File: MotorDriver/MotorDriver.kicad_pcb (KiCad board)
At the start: 2 copper layers, 78 x 48.6 mm, 47 parts, among them J1 VIN, J2 INPUT, M1 Motor_DC, Q1 Q_NMOS_GDS, Q2 Q_NMOS_GDS, Q3 Q_NMOS_GDS, Q4 Q_NMOS_GDS, U1 IR2302, U2 IR2302, U3 74HC00, U4 TLP2348, U5 TLP2348, U6 NJM7812SDL1

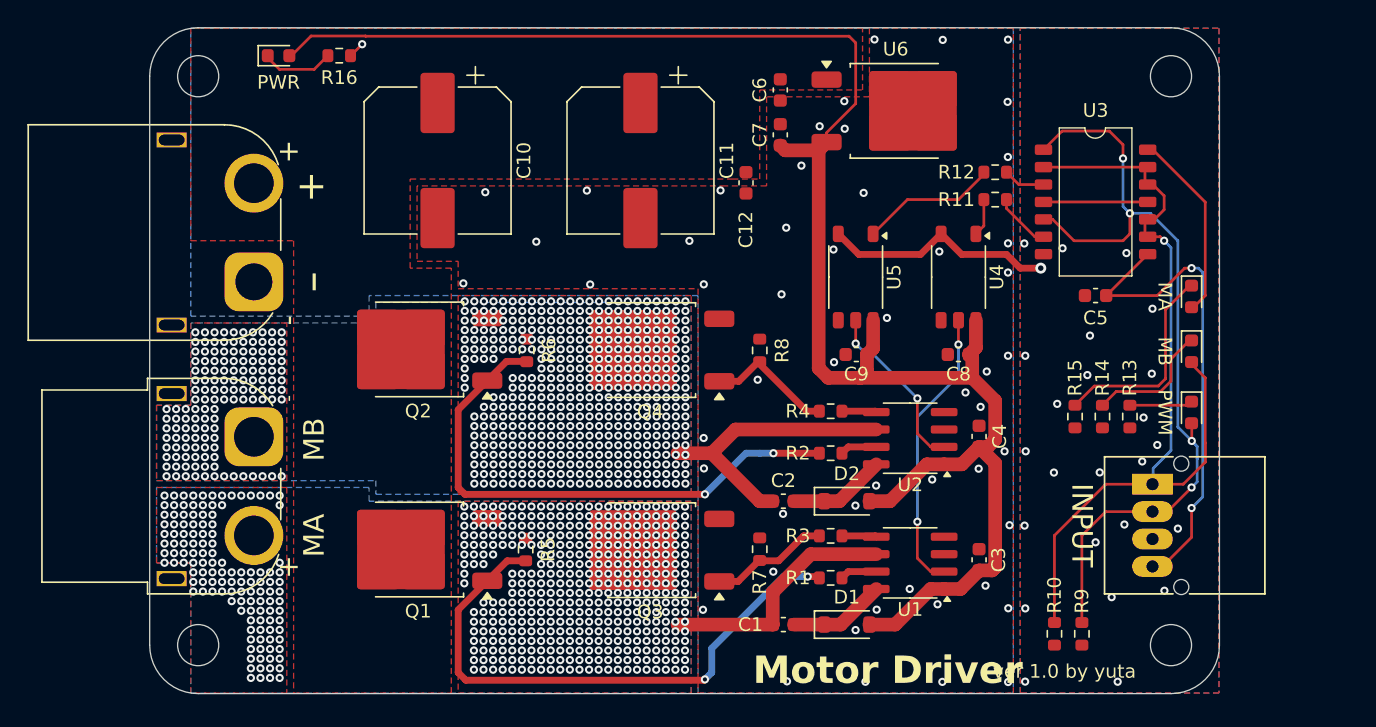
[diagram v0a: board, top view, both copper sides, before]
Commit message: Motor Driver ver2.0
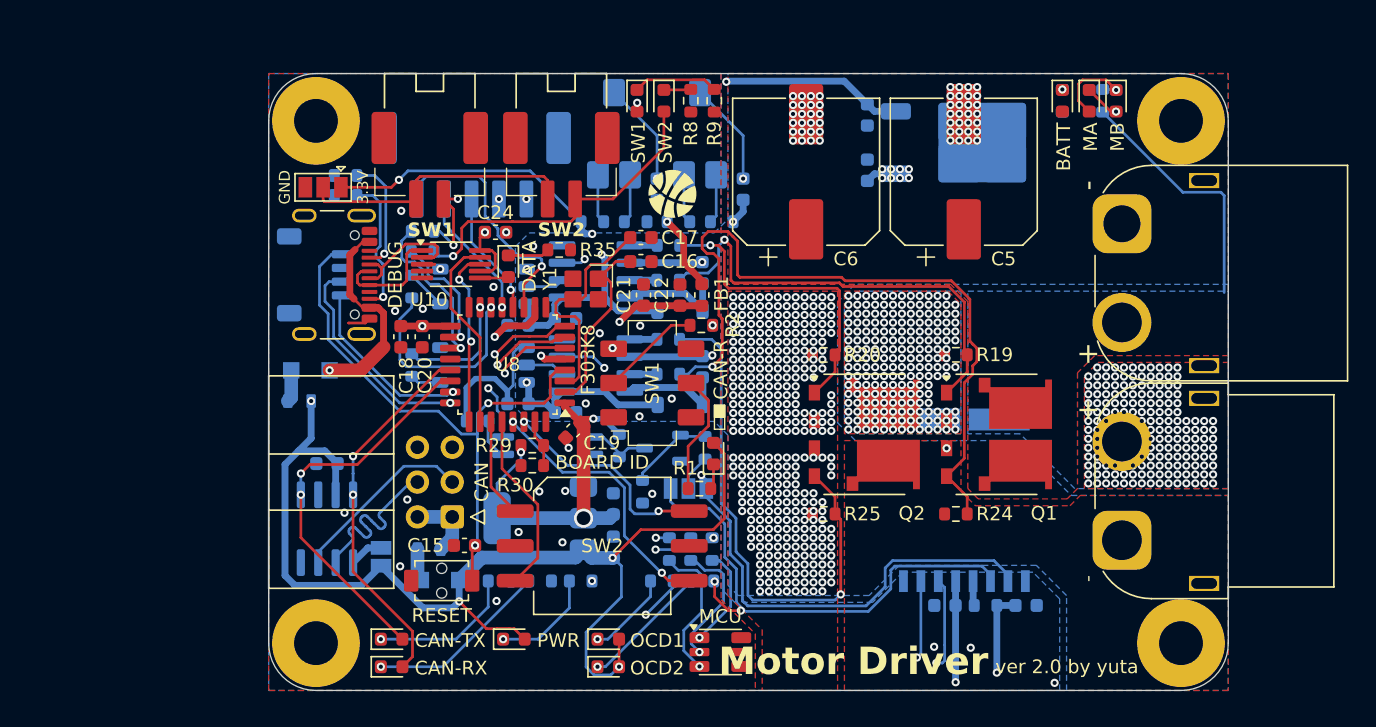
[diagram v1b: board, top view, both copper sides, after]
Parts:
- removed M1: Motor_DC, Anan-Robo_Footprint_Library:XT60PW-F_Horizontal
- removed Q4: Q_NMOS_GDS, Package_TO_SOT_SMD:TO-252-2
- added C13: 2.5u, Capacitor_SMD:C_0603_1608Metric, B.Cu at (150.1, 100.5)
- added C14: 0.1u, Capacitor_SMD:C_0603_1608Metric, B.Cu at (140.2, 103.8)
- added C15: 0.1u, Capacitor_SMD:C_0603_1608Metric, F.Cu at (132.8, 113.5)
- added C16: 15p, Capacitor_SMD:C_0603_1608Metric, F.Cu at (145.7, 92.8)
- added C17: 15p, Capacitor_SMD:C_0603_1608Metric, F.Cu at (145.7, 91.1)
- added C18: 4.7u, Capacitor_SMD:C_0603_1608Metric, F.Cu at (128.1, 98.3)
- added C19: 0.1u, Capacitor_SMD:C_0603_1608Metric, F.Cu at (140.7, 105.2)
- added C20: 0.1u, Capacitor_SMD:C_0603_1608Metric, F.Cu at (129.7, 98.3)
- added C21: 0.1u, Capacitor_SMD:C_0603_1608Metric, F.Cu at (145.8, 95.3)
- added C22: 1u, Capacitor_SMD:C_0603_1608Metric, F.Cu at (148.5, 95.3)
- added C23: 0.1u, Capacitor_SMD:C_0603_1608Metric, B.Cu at (122.8, 107.6)
- added C24: 0.1u, Capacitor_SMD:C_0603_1608Metric, F.Cu at (135.1, 90.7)
- added C25: 0.1u, Capacitor_SMD:C_0603_1608Metric, B.Cu at (136.7, 97.5)
- added C26: 0.1u, Capacitor_SMD:C_0603_1608Metric, B.Cu at (136.7, 103.2)
- added D10: OCD1, LED_SMD:LED_0603_1608Metric, F.Cu at (143.3, 120.4)
- added D11: OCD2, LED_SMD:LED_0603_1608Metric, F.Cu at (143.3, 122.4)
- added D12: D_Schottky, Diode_SMD:D_SOD-123, B.Cu at (148.5, 103.3)
- added D13: CAN_TX, LED_SMD:LED_0603_1608Metric, F.Cu at (127.5, 120.4)
- added D14: CAN_RX, LED_SMD:LED_0603_1608Metric, F.Cu at (127.5, 122.4)
- added D15: D, Diode_SMD:Nexperia_CFP3_SOD-123W, B.Cu at (121.5, 100.8)
- added D16: DATA, LED_SMD:LED_0603_1608Metric, F.Cu at (136.0, 93.2)
- added D7: D_Schottky, Diode_SMD:D_SOD-123, B.Cu at (148.5, 96.4)
- added D8: MA, LED_SMD:LED_0603_1608Metric, F.Cu at (178.4, 81.1)
- added D9: MB, LED_SMD:LED_0603_1608Metric, F.Cu at (180.3, 81.1)
- added F1: Polyfuse, Anan-Robo_Footprint_Library:MF-FSMF, B.Cu at (130.2, 113.8)
- added F2: Polyfuse, Anan-Robo_Footprint_Library:MF-FSMF, B.Cu at (120.7, 103.0)
- added FB1: FerriteBead, Inductor_SMD:L_0603_1608Metric, F.Cu at (150.1, 95.3)
- added G***: LOGO, LOGO, F.Cu at (147.9, 87.9)
- added H1: MountingHole_Pad, MountingHole:MountingHole_3.2mm_M3_Pad, F.Cu at (122.0, 82.6)
- added H2: MountingHole_Pad, MountingHole:MountingHole_3.2mm_M3_Pad, F.Cu at (122.0, 120.7)
- added H3: MountingHole_Pad, MountingHole:MountingHole_3.2mm_M3_Pad, F.Cu at (185.1, 82.6)
- added H4: MountingHole_Pad, MountingHole:MountingHole_3.2mm_M3_Pad, F.Cu at (185.1, 120.7)
- added H5: MountingHole, Anan-Robo_Footprint_Library:Title, F.Cu at (77.9, 108.2)
- added H6: MountingHole, Anan-Robo_Footprint_Library:Aho_old_S, B.Cu at (169.9, 94.6)
- added H7: MountingHole, Anan-Robo_Footprint_Library:Aho_new_S, B.Cu at (158.4, 94.6)
- added H8: MountingHole, Anan-Robo_Footprint_Library:Info_M_3, B.Cu at (158.4, 107.3)
- added J3: SW1, Anan-Robo_Footprint_Library:SM02B-PASS-TBx, F.Cu at (130.2, 84.4)
- added J4: SW2, Anan-Robo_Footprint_Library:SM02B-PASS-TBx, F.Cu at (139.8, 84.4)
- added J5: VIN, Anan-Robo_Footprint_Library:XT60PW-M_Horizontal, F.Cu at (189.5, 93.8)
- added J6: Motor, Anan-Robo_Footprint_Library:XT60PW-F_Horizontal, F.Cu at (186.7, 109.8)
- added J7: SWD, Connector_JST:JST_SH_SM04B-SRSS-TB_1x04-1MP_P1.00mm_Horizontal, B.Cu at (121.9, 93.8)
- added J8: Debug, Connector_USB:USB_C_Receptacle_GCT_USB4105-xx-A_16P_TopMnt_Horizontal, F.Cu at (122.2, 93.8)
- added JP1: Up/Down, Jumper:SolderJumper-3_P1.3mm_Open_Pad1.0x1.5mm, F.Cu at (122.5, 87.4)
- added JP2: OCD, Jumper:SolderJumper-3_P1.3mm_Open_Pad1.0x1.5mm, B.Cu at (149.1, 109.4)
- added JP4: MCP2561/2FD selector, Jumper:SolderJumper-2_P1.3mm_Open_Pad1.0x1.5mm, B.Cu at (126.7, 114.4)
- added R17: 80, Resistor_SMD:R_0603_1608Metric, B.Cu at (147.7, 91.7)
- added R18: 1.5k, Resistor_SMD:R_0603_1608Metric, B.Cu at (170.8, 117.9)
- added R19: 10k, Resistor_SMD:R_0603_1608Metric, F.Cu at (168.6, 99.6)
- added R20: 10k, Resistor_SMD:R_0603_1608Metric, F.Cu at (159.0, 99.7)
- added R21: 3.7k, Resistor_SMD:R_0603_1608Metric, B.Cu at (179.3, 81.1)
- added R22: 420, Resistor_SMD:R_0603_1608Metric, B.Cu at (147.2, 116.1)
- added R23: 420, Resistor_SMD:R_0603_1608Metric, B.Cu at (150.1, 116.1)
- added R24: 10k, Resistor_SMD:R_0603_1608Metric, F.Cu at (168.6, 111.2)
- added R25: 10k, Resistor_SMD:R_0603_1608Metric, F.Cu at (159.0, 111.2)
- added R26: 80, Resistor_SMD:R_0603_1608Metric, B.Cu at (147.7, 101.1)
- added R27: 80, Resistor_SMD:R_0603_1608Metric, B.Cu at (147.6, 98.5)
- added R28: 1k, Resistor_SMD:R_0603_1608Metric, B.Cu at (144.1, 106.3)
- added R29: 10k, Resistor_SMD:R_0603_1608Metric, F.Cu at (137.7, 106.3)
- added R30: 10k, Resistor_SMD:R_0603_1608Metric, F.Cu at (137.7, 107.7)
- added R31: 100, Resistor_SMD:R_0603_1608Metric, B.Cu at (135.3, 116.1)
- added R32: 100, Resistor_SMD:R_0603_1608Metric, B.Cu at (138.3, 116.1)
- added R33: 5.1k, Resistor_SMD:R_0603_1608Metric, B.Cu at (124.1, 88.0)
- added R34: 5.1k, Resistor_SMD:R_0603_1608Metric, B.Cu at (124.1, 86.6)
- added R35: 100, Resistor_SMD:R_0603_1608Metric, F.Cu at (139.7, 92.0)
- added R36: 350, Resistor_SMD:R_0603_1608Metric, B.Cu at (128.9, 94.7)
- added R37: 350, Resistor_SMD:R_0603_1608Metric, B.Cu at (128.9, 100.4)
- added R38: 660, Resistor_SMD:R_0603_1608Metric, B.Cu at (150.3, 106.4)
- added R39: 10k, Resistor_SMD:R_0603_1608Metric, B.Cu at (145.8, 109.6)
- added R40: 10k, Resistor_SMD:R_0603_1608Metric, B.Cu at (133.7, 104.5)
- added RV1: 10k, Anan-Robo_Footprint_Library:ST-4ETB103, B.Cu at (150.0, 83.5)
- added RV2: 10k, Anan-Robo_Footprint_Library:ST-4ETB103, B.Cu at (143.7, 83.5)
- added SW1: CAN_R, Anan-Robo_Footprint_Library:SLW, F.Cu at (146.5, 101.7)
- added SW2: SW_Coded, Anan-Robo_Footprint_Library:RDS-1055-SMT, F.Cu at (142.8, 113.6)
- added SW3: RESET, Anan-Robo_Footprint_Library:TVAF06-A020B-R, F.Cu at (131.1, 116.1)
- added U10: CH340E, Package_SO:MSOP-10_3x3mm_P0.5mm, F.Cu at (131.8, 93.0)
- added U11: TLP2348, Package_SO:SO-5-6_4.55x3.7mm_P1.27mm, B.Cu at (134.2, 94.7)
- added U12: TLP2348, Package_SO:SO-5-6_4.55x3.7mm_P1.27mm, B.Cu at (134.2, 100.4)
- added U7: TLP293, Package_SO:SOIC-4_4.55x2.6mm_P1.27mm, B.Cu at (138.8, 106.3)
- added U8: STM32F303K8Tx, Package_QFP:LQFP-32_7x7mm_P0.8mm, F.Cu at (135.9, 100.3)
- added U9: MCP2561/2FD, Package_SO:SOIC-8_3.9x4.9mm_P1.27mm, B.Cu at (122.8, 112.3)
- added Y1: Crystal_GND2, Anan-Robo_Footprint_Library:XRCGB, F.Cu at (141.6, 94.8)
- C1: value 10u -> 0.33u; moved to B.Cu
- C10: value 330u -> 2.5u; footprint Capacitor_SMD:CP_Elec_10x10.5 -> Capacitor_SMD:C_0603_1608Metric; moved to B.Cu
- C11: value 330u -> 1000p; footprint Capacitor_SMD:CP_Elec_10x10.5 -> Capacitor_SMD:C_0603_1608Metric; moved to B.Cu
- C12: value 1u -> 1000p; moved to B.Cu
- C2: value 10u -> 4.7u; moved to B.Cu
- C3, C7, C9: moved to B.Cu
- C4: value 0.1u -> 4.7u; moved to B.Cu
- C5: value 0.1u -> 330u; footprint Capacitor_SMD:C_0603_1608Metric -> Capacitor_SMD:CP_Elec_10x10.5
- C6: value 0.33u -> 330u; footprint Capacitor_SMD:C_0603_1608Metric -> Capacitor_SMD:CP_Elec_10x10.5
- C8: value 0.1u -> 1000p; moved to B.Cu
- D1: value D_Schottky -> D; footprint Diode_SMD:D_SOD-123 -> Diode_SMD:Nexperia_CFP3_SOD-123W; moved to B.Cu
- D2: value D_Schottky -> CAN_R; footprint Diode_SMD:D_SOD-123 -> LED_SMD:LED_0603_1608Metric
- D3: value PWM -> SW2
- D4: value MA -> SW1
- D5: value MB -> PWR
- D6: value PWR -> BATT
- J1: value VIN -> CAN; footprint Anan-Robo_Footprint_Library:XT60PW-M_Horizontal -> Connector_IDC:IDC-Header_2x03_P2.54mm_Horizontal
- J2: value INPUT -> ENC; footprint Anan-Robo_Footprint_Library:PAコネクタ(4ピンサイド型) -> Anan-Robo_Footprint_Library:SM05B-PASS-TBx; moved to B.Cu
- Q1, Q2: value Q_NMOS_GDS -> Q_NMOS; footprint Package_TO_SOT_SMD:TO-252-2 -> Anan-Robo_Footprint_Library:Vishay_PowerPAK_8x8L_Dual
- Q3: value Q_NMOS_GDS -> Q_NMOS_GSD; footprint Package_TO_SOT_SMD:TO-252-2 -> Package_TO_SOT_SMD:TSOT-23; moved to B.Cu
- R1: value 80 -> 420
- R10: value 20k -> 430; moved to B.Cu
- R11: value 175 -> 1.5k; moved to B.Cu
- R12: value 175 -> 13k; moved to B.Cu
- R13: value 80 -> 2.4k; moved to B.Cu
- R14: value 80 -> 18k; moved to B.Cu
- R15: value 80 -> 3k; moved to B.Cu
- R16: value 500 -> 80; moved to B.Cu
- R2: value 80 -> 120
- R3: value 80 -> 100; moved to B.Cu
- R4: value 80 -> 600; moved to B.Cu
- R5: value 20k -> 300; moved to B.Cu
- R6, R7: value 20k -> 330; moved to B.Cu
- R8, R9: value 20k -> 80
- U1: value IR2302 -> LED_GRB; footprint Package_SO:SOIC-8_3.9x4.9mm_P1.27mm -> LED_SMD:LED_ROHM_SMLVN6
- U2: value IR2302 -> NJM7812SDL1; footprint Package_SO:SOIC-8_3.9x4.9mm_P1.27mm -> Package_TO_SOT_SMD:TO-252-2; moved to B.Cu
- U3: value 74HC00 -> TLV1117-33; footprint Anan-Robo_Footprint_Library:SOP14 -> Package_TO_SOT_SMD:SOT-223-3_TabPin2; moved to B.Cu
- U4: value TLP2348 -> CZ-3A05; footprint Package_SO:SO-5-6_4.55x3.7mm_P1.27mm -> Anan-Robo_Footprint_Library:CZ3A; moved to B.Cu
- U5: value TLP2348 -> IR2302; footprint Package_SO:SO-5-6_4.55x3.7mm_P1.27mm -> Package_SO:SOIC-8_3.9x4.9mm_P1.27mm; moved to B.Cu
- U6: value NJM7812SDL1 -> IR2302; footprint Package_TO_SOT_SMD:TO-252-2 -> Package_SO:SOIC-8_3.9x4.9mm_P1.27mm; moved to B.Cu
- moved J2 57.3 mm to (133.3, 83.6), turned to 180 degrees
- moved D6 57.3 mm to (176.4, 81.1), turned to -90 degrees
- moved D5 53.7 mm to (136.4, 120.4), turned to 0 degrees
- moved U3 50.4 mm to (138.3, 111.6), turned to 180 degrees
- moved R9 47.2 mm to (151.0, 81.1)
- moved D3 44.7 mm to (147.3, 81.1)
- moved Q1 43.0 mm to (171.6, 105.4), turned to 0 degrees
- moved D4 42.9 mm to (145.4, 81.1)
- moved R14 39.8 mm to (142.1, 89.9), turned to 0 degrees
- moved C12 37.0 mm to (173.8, 117.9), turned to 0 degrees
- moved C7 36.4 mm to (167.8, 117.9), turned to 180 degrees
- moved R15 35.1 mm to (145.3, 89.9), turned to 0 degrees
- moved R10 34.8 mm to (141.3, 116.1), turned to 0 degrees
- moved C1 33.7 mm to (162.2, 86.2), turned to 90 degrees
- moved C3 33.5 mm to (162.2, 82.1)
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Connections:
- C1 pad 1: Net-(D1-K) -> +BATT
- C1 pad 2: /MA -> GNDA
- C10 pad 1: +24V -> Net-(D7-K)
- C10 pad 2: GNDPWR -> CS+
- C11 pad 1: +24V -> REF2
- C11 pad 2: GNDPWR -> GNDD
- C12 pad 1: +24V -> /Driver/VOUT
- C12 pad 2: GNDPWR -> GNDD
- C2 pad 1: Net-(D2-K) -> +5VD
- C2 pad 2: /MB -> GNDD
- C3 pad 1: GNDPWR -> +12VA
- C3 pad 2: +12V -> GNDA
- C4 pad 1: +12V -> +3.3VD
- C4 pad 2: GNDPWR -> GNDD
- C5 pad 1: GND -> +BATT
- C5 pad 2: +3V3 -> GNDA
- C6 pad 1: +24V -> +BATT
- C6 pad 2: GNDPWR -> GNDA
- C7 pad 1: +12V -> +3.3VD
- C7 pad 2: GNDPWR -> GNDD
- C8 pad 1: +12V -> REF1
- C8 pad 2: GNDPWR -> GNDD
- C9 pad 1: +12V -> GNDA
- C9 pad 2: GNDPWR -> +12VA
- D1 pad 1: Net-(D1-K) -> +5VD
- D1 pad 2: +12V -> Net-(D1-A)
- D2 pad 2: +12V -> +5VD
- D3 pad 2: PWM -> Net-(D3-A)
- D5 pad 2: DIR -> +5VD
- D6 pad 2: +12V -> +BATT
- J1 pad 1: +24V -> Net-(J1-Pin_1)
- J1 pad 2: GNDPWR -> Net-(J1-Pin_1)
- J2 pad 1: +3V3 -> /MCU/X/SCK
- J2 pad 2: GND -> /MCU/ENC_B/DATA
- J2 pad 3: PWM -> /MCU/ENC_A/MISO
- J2 pad 4: DIR -> +5VD
- Q1 pad 1: Net-(Q1-G) -> Net-(Q1A-G)
- Q1 pad 2: +24V -> CS+
- Q1 pad 3: /MA -> /Driver/MB
- Q2 pad 1: Net-(Q2-G) -> Net-(Q2A-G)
- Q2 pad 2: +24V -> GNDA
- Q2 pad 3: /MB -> GNDA
- Q3 pad 2: /MA -> GNDD
- Q3 pad 3: GNDPWR -> Net-(Q3-D)
- R1 pad 1: Net-(Q1-G) -> Net-(D2-K)
- R1 pad 2: Net-(U1-HO) -> Net-(SW1B-B)
- R10 pad 1: DIR -> Net-(D5-K)
- R10 pad 2: GND -> GNDD
- R11 pad 1: Net-(U4-A) -> Net-(D6-K)
- R11 pad 2: /_INPUT1 -> GNDA
- R12 pad 1: Net-(U5-A) -> +3.3VD
- R12 pad 2: /_INPUT2 -> Net-(R12-Pad2)
- R13 pad 1: GND -> Net-(R13-Pad1)
- R13 pad 2: Net-(D3-K) -> GNDD
- R14 pad 1: GND -> +3.3VD
- R14 pad 2: Net-(D5-K) -> Net-(R14-Pad2)
- R15 pad 1: GND -> Net-(R15-Pad1)
- R15 pad 2: Net-(D4-K) -> GNDD
- R16 pad 1: Net-(D6-K) -> Net-(Q1A-G)
- R16 pad 2: GNDPWR -> Net-(U5-HO)
- R2 pad 1: Net-(U2-HO) -> /CAN/CAN_H
- R2 pad 2: Net-(Q2-G) -> Net-(SW1A-B)
- R3 pad 1: Net-(Q3-G) -> Net-(R3-Pad1)
- R3 pad 2: Net-(U1-LO) -> /MCU/LED_R
- R4 pad 1: Net-(U2-LO) -> Net-(R4-Pad1)
- R4 pad 2: Net-(Q4-G) -> /MCU/LED_B
- R5 pad 1: Net-(Q1-G) -> Net-(R5-Pad1)
- R5 pad 2: /MA -> /MCU/LED_G
- R6 pad 1: Net-(Q2-G) -> /MCU/SW1
- R6 pad 2: /MB -> Net-(D4-A)
- R7 pad 1: Net-(Q3-G) -> /MCU/SW2
- R7 pad 2: GNDPWR -> Net-(D3-A)
- R8 pad 1: Net-(Q4-G) -> Net-(D3-K)
- R8 pad 2: GNDPWR -> GNDD
- R9 pad 1: PWM -> Net-(D4-K)
- R9 pad 2: GND -> GNDD
- U1 pad 1: +12V -> Net-(R3-Pad1)
- U1 pad 2: INPUT1 -> Net-(R4-Pad1)
- U1 pad 3: unconnected-(U1-~{SD}-Pad3) -> Net-(R5-Pad1)
- U1 pad 4: GNDPWR -> GNDD
- U1 pad 5: Net-(U1-LO) -> GNDD
- U1 pad 6: /MA -> GNDD
- U2 pad 1: +12V -> +BATT
- U2 pad 2: INPUT2 -> GNDA
- U2 pad 3: unconnected-(U2-~{SD}-Pad3) -> +12VA
- U3 pad 1: PWM -> GNDD
- U3 pad 2: DIR -> +3.3VD
- U3 pad 3: /_INPUT2 -> +5VD
- U4 pad 1: Net-(U4-A) -> GNDD
- U4 pad 3: GND -> OCD2
- U4 pad 4: GNDPWR -> Net-(U4-VOUT)
- U4 pad 5: INPUT1 -> +3.3VD
- U4 pad 6: +12V -> REF1
- U5 pad 1: Net-(U5-A) -> +12VA
- U5 pad 3: GND -> SD
- U5 pad 4: GNDPWR -> GNDA
- U5 pad 5: INPUT2 -> Net-(U5-LO)
- U5 pad 6: +12V -> CS+
- U6 pad 1: +24V -> +12VA
- U6 pad 2: GNDPWR -> /Driver/INPUT2
- U6 pad 3: +12V -> SD
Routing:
- net +3.3VD: track 0.00 -> 157.7 mm, vias 0 -> 9
- net +12V: track 127.6 -> 0.00 mm
- net +5VD: track 0.00 -> 106.5 mm, vias 0 -> 5
- net /Driver/MB: track 0.00 -> 72.8 mm, vias 0 -> 3
- net REF2: track 0.00 -> 72.7 mm, vias 0 -> 2
- net +12VA: track 0.00 -> 71.8 mm, vias 0 -> 3
- net REF1: track 0.00 -> 68.2 mm, vias 0 -> 2
- net /Driver/VOUT: track 0.00 -> 67.9 mm, vias 0 -> 2
- net DIR: track 61.6 -> 0.00 mm, vias 1 -> 0
- net PWM: track 61.1 -> 0.00 mm, vias 4 -> 0
- net Net-(Q1B-G): track 0.00 -> 53.8 mm, vias 0 -> 1
- net OCD1: track 0.00 -> 48.2 mm, vias 0 -> 2
- net /MCU/NRST: track 0.00 -> 42.3 mm, vias 0 -> 2
- net Net-(Q1-G): track 41.8 -> 0.00 mm, vias 2 -> 0
- net Net-(Q2-G): track 39.9 -> 0.00 mm, vias 2 -> 0
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- added copper zone on F.Cu, net +BATT
- added copper zone on In1.Cu, net +BATT
- added copper zone on F.Cu, net /Driver/MB
- added copper zone on In1.Cu, net /Driver/MB
- added copper zone on B.Cu, net CS+
- added copper zone on F.Cu, net CS+
- added copper zone on In1.Cu, net CS+
- added copper zone on B.Cu, net CS-
- added copper zone on F.Cu, net CS-
- added copper zone on In1.Cu, net CS-
- added copper zone on In2.Cu, net CS-
- added copper zone on B.Cu, net GNDA
- added copper zone on F.Cu, net GNDA
- added copper zone on In2.Cu, net GNDA
- added copper zone on B.Cu, net GNDD
- added copper zone on F.Cu, net GNDD
- added copper zone on In1.Cu, net GNDD
- added copper zone on In2.Cu, net GNDD
- removed copper zone on F.Cu, net +24V
- removed copper zone on B.Cu, net /MA
- removed copper zone on F.Cu, net /MA
- removed copper zone on B.Cu, net /MB
- removed copper zone on F.Cu, net /MB
- removed copper zone on B.Cu, net GND
- removed copper zone on F.Cu, net GND
- removed copper zone on B.Cu, net GNDPWR
- removed copper zone on F.Cu, net GNDPWR
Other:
- board size 78 x 48.6 mm -> 70 x 45 mm
- copper layers 2 -> 4
- board text added: "-"
- board text added: "5V"
- board text added: "ADJ1"
- board text added: "ADJ2"
- board text added: "BATT"
- board text added: "BOARD ID"
- board text added: "CAN"
- board text added: "CAN-H"
- board text added: "CAN-L"
- board text added: "CAN-R"
- board text added: "CAN-RX"
- board text added: "CAN-TX"
- board text added: "DATA"
- board text added: "DEBUG"
- board text added: "ENC"
- board text added: "F303K8"
- board text added: "MCU"
- board text added: "OCD"
- board text added: "OCD1"
- board text added: "OCD2"
- board text added: "R13 R12 R15 R14"
- board text added: "RESET"
- board text added: "SW1"
- board text added: "SW2"
- board text added: "SWD"
- board text added: "ver 2.0: 2025-07-11"
- board text removed: "DATE"
- board text removed: "DIR"
- board text removed: "INPUT"
- board text removed: "Motor Driver"
- board text removed: "No."
- board text removed: "PWM"
- board text removed: "TEST"
- board text removed: "VOLTAGE: 12~24V CURRENT: 30A"
- board text removed: "_"
- board text removed: "ver 1.0 by yuta"
